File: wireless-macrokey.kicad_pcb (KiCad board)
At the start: 2 copper layers, 110.3 x 93.4 mm, 25 parts, among them J1 ENC0, J2 ENC1, J3 ENC2, J4 OLED, J5 POWER 5V, J6 SERIAL, J7 LED, SW1 SW_Push_45deg, SW10 SW_Push_45deg, SW11 SW_Push_45deg, SW12 SW_Push_45deg, SW13 SW_Push_45deg, SW14 SW_Push_45deg, SW2 SW_Push_45deg, SW3 SW_Push_45deg, SW4 SW_Push_45deg, SW5 SW_Push_45deg, SW6 SW_Push_45deg, SW7 SW_Push_45deg, SW8 SW_Push_45deg, SW9 SW_Push_45deg, U1 ESP32-WROOM-32E, U3 LM1117T-3.3

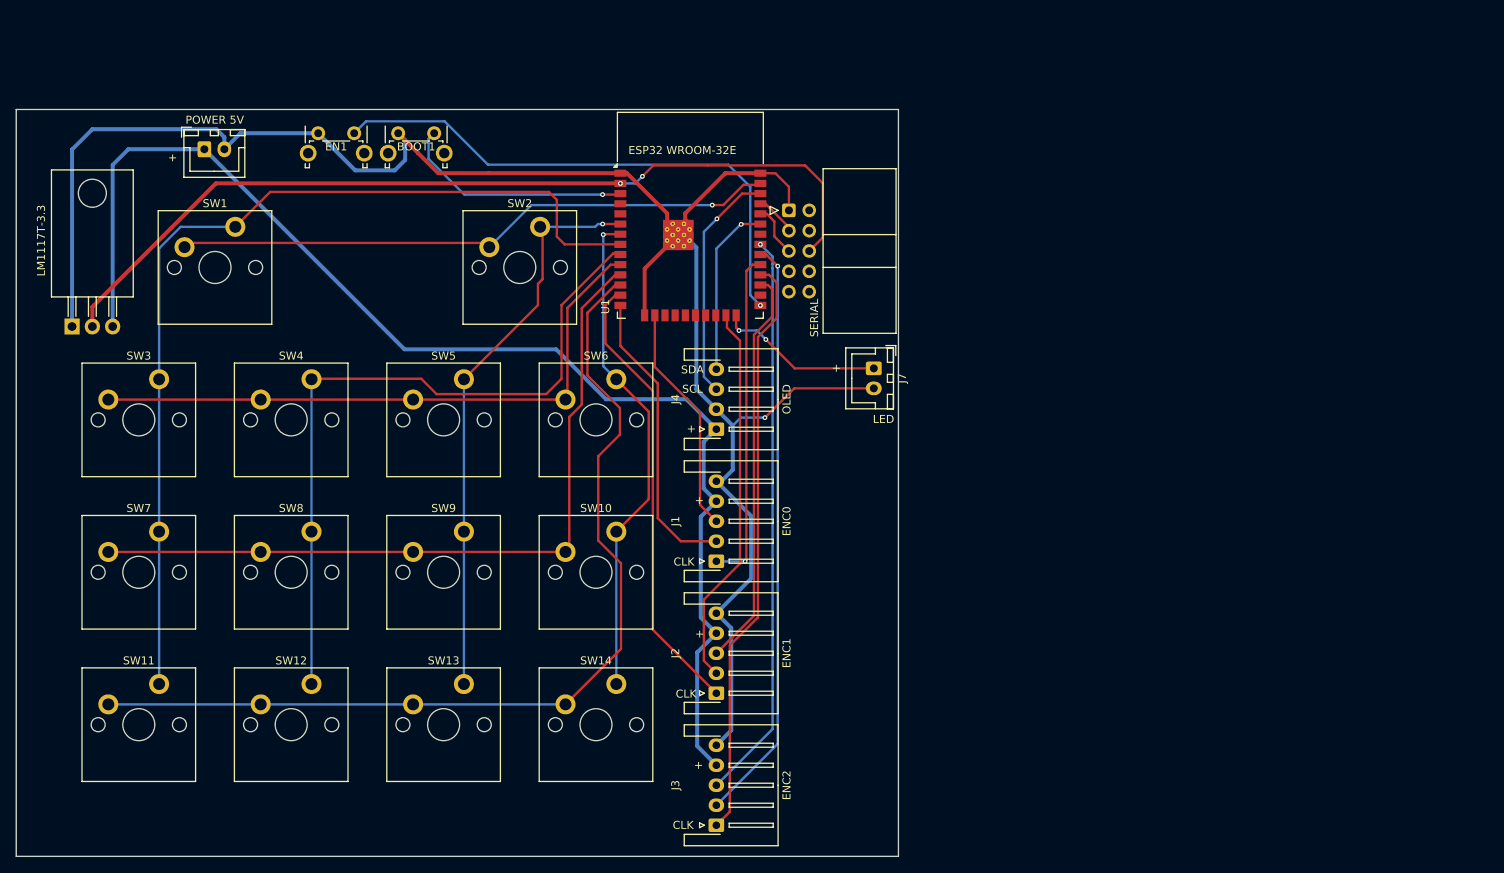
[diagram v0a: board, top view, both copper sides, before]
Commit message: x
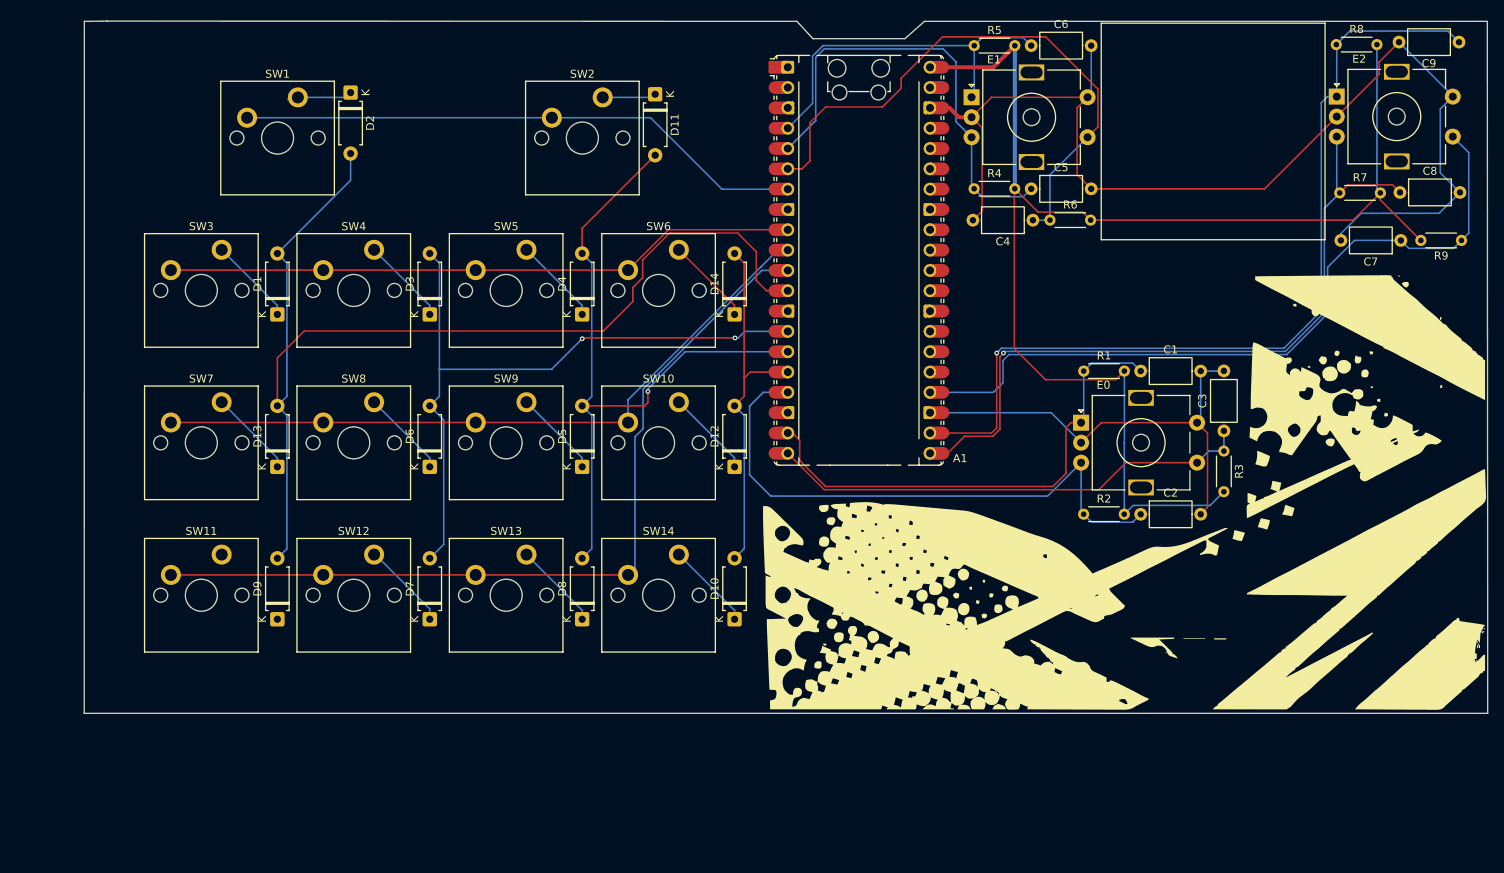
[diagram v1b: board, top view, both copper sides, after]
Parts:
- removed BOOT1, EN1: SW_Push, Button_Switch_THT:SW_Tactile_SPST_Angled_PTS645Vx39-2LFS
- removed J1: ENC0, Connector_JST:JST_XH_S5B-XH-A-1_1x05_P2.50mm_Horizontal
- removed J2: ENC1, Connector_JST:JST_XH_S5B-XH-A-1_1x05_P2.50mm_Horizontal
- removed J3: ENC2, Connector_JST:JST_XH_S5B-XH-A-1_1x05_P2.50mm_Horizontal
- removed J4: OLED, Connector_JST:JST_XH_S4B-XH-A-1_1x04_P2.50mm_Horizontal
- removed J5: POWER 5V, Connector_JST:JST_XH_B2B-XH-A_1x02_P2.50mm_Vertical
- removed J6: SERIAL, Connector_IDC:IDC-Header_2x05_P2.54mm_Horizontal
- removed J7: LED, Connector_JST:JST_XH_B2B-XH-A_1x02_P2.50mm_Vertical
- removed U1: ESP32-WROOM-32E, RF_Module:ESP32-WROOM-32D
- removed U3: LM1117T-3.3, Package_TO_SOT_THT:TO-220-3_Horizontal_TabDown
- added A1: RaspberryPi_Pico, Module:RaspberryPi_Pico_Common_Unspecified, F.Cu at (129.8, 53.4)
- added C1: 1uF, Capacitor_THT:C_Axial_L5.1mm_D3.1mm_P7.50mm_Horizontal, F.Cu at (165.0, 67.2)
- added C2: 1uF, Capacitor_THT:C_Axial_L5.1mm_D3.1mm_P7.50mm_Horizontal, F.Cu at (165.0, 85.1)
- added C3: 1uF, Capacitor_THT:C_Axial_L5.1mm_D3.1mm_P7.50mm_Horizontal, F.Cu at (175.4, 74.7)
- added C4: 1uF, Capacitor_THT:C_Axial_L5.1mm_D3.1mm_P7.50mm_Horizontal, F.Cu at (151.6, 48.4)
- added C5: 1uF, Capacitor_THT:C_Axial_L5.1mm_D3.1mm_P7.50mm_Horizontal, F.Cu at (151.3, 44.5)
- added C6: 1uF, Capacitor_THT:C_Axial_L5.1mm_D3.1mm_P7.50mm_Horizontal, F.Cu at (151.3, 26.6)
- added C7: 1uF, Capacitor_THT:C_Axial_L5.1mm_D3.1mm_P7.50mm_Horizontal, F.Cu at (197.6, 50.9)
- added C8: 1uF, Capacitor_THT:C_Axial_L5.1mm_D3.1mm_P7.50mm_Horizontal, F.Cu at (197.4, 44.9)
- added C9: 1uF, Capacitor_THT:C_Axial_L5.1mm_D3.1mm_P7.50mm_Horizontal, F.Cu at (204.8, 26.1)
- added D1: D_45deg, Diode_THT:D_A-405_P7.62mm_Horizontal, F.Cu at (57.1, 60.1)
- added D10: D_45deg, Diode_THT:D_A-405_P7.62mm_Horizontal, F.Cu at (114.3, 98.2)
- added D11: D_45deg, Diode_THT:D_A-405_P7.62mm_Horizontal, F.Cu at (104.3, 32.6)
- added D12: D_45deg, Diode_THT:D_A-405_P7.62mm_Horizontal, F.Cu at (114.3, 79.2)
- added D13: D_45deg, Diode_THT:D_A-405_P7.62mm_Horizontal, F.Cu at (57.1, 79.2)
- added D14: D_45deg, Diode_THT:D_A-405_P7.62mm_Horizontal, F.Cu at (114.3, 60.1)
- added D2: D_45deg, Diode_THT:D_A-405_P7.62mm_Horizontal, F.Cu at (66.3, 32.4)
- added D3: D_45deg, Diode_THT:D_A-405_P7.62mm_Horizontal, F.Cu at (76.2, 60.1)
- added D4: D_45deg, Diode_THT:D_A-405_P7.62mm_Horizontal, F.Cu at (95.2, 60.1)
- added D5: D_45deg, Diode_THT:D_A-405_P7.62mm_Horizontal, F.Cu at (95.2, 79.2)
- added D6: D_45deg, Diode_THT:D_A-405_P7.62mm_Horizontal, F.Cu at (76.2, 79.2)
- added D7: D_45deg, Diode_THT:D_A-405_P7.62mm_Horizontal, F.Cu at (76.2, 98.2)
- added D8: D_45deg, Diode_THT:D_A-405_P7.62mm_Horizontal, F.Cu at (95.2, 98.2)
- added D9: D_45deg, Diode_THT:D_A-405_P7.62mm_Horizontal, F.Cu at (57.1, 98.2)
- added E0: RotaryEncoder_Switch_MP, Rotary_Encoder:RotaryEncoder_Alps_EC11E-Switch_Vertical_H20mm_MountingHoles, F.Cu at (157.6, 73.7)
- added E1: RotaryEncoder_Switch_MP, Rotary_Encoder:RotaryEncoder_Alps_EC11E-Switch_Vertical_H20mm_MountingHoles, F.Cu at (143.9, 33.0)
- added E2: RotaryEncoder_Switch_MP, Rotary_Encoder:RotaryEncoder_Alps_EC11E-Switch_Vertical_H20mm_MountingHoles, F.Cu at (189.6, 32.9)
- added R1: 1k, Resistor_THT:R_Axial_DIN0204_L3.6mm_D1.6mm_P5.08mm_Horizontal, F.Cu at (157.9, 67.2)
- added R2: 1k, Resistor_THT:R_Axial_DIN0204_L3.6mm_D1.6mm_P5.08mm_Horizontal, F.Cu at (157.9, 85.1)
- added R3: 1k, Resistor_THT:R_Axial_DIN0204_L3.6mm_D1.6mm_P5.08mm_Horizontal, F.Cu at (175.4, 77.2)
- added R4: 1k, Resistor_THT:R_Axial_DIN0204_L3.6mm_D1.6mm_P5.08mm_Horizontal, F.Cu at (144.2, 44.4)
- added R5: 1k, Resistor_THT:R_Axial_DIN0204_L3.6mm_D1.6mm_P5.08mm_Horizontal, F.Cu at (144.2, 26.6)
- added R6: 1k, Resistor_THT:R_Axial_DIN0204_L3.6mm_D1.6mm_P5.08mm_Horizontal, F.Cu at (153.7, 48.4)
- added R7: 1k, Resistor_THT:R_Axial_DIN0204_L3.6mm_D1.6mm_P5.08mm_Horizontal, F.Cu at (189.9, 45.0)
- added R8: 1k, Resistor_THT:R_Axial_DIN0204_L3.6mm_D1.6mm_P5.08mm_Horizontal, F.Cu at (189.5, 26.4)
- added R9: 1k, Resistor_THT:R_Axial_DIN0204_L3.6mm_D1.6mm_P5.08mm_Horizontal, F.Cu at (205.1, 50.9)
- SW1, SW2: footprint PCM_Switch_Keyboard_Cherry_MX:SW_Cherry_MX_PCB_1.00u -> PCM_Switch_Keyboard_Cherry_MX:SW_Cherry_MX_PCB_2.00u
- moved SW14 18.0 mm to (104.8, 95.2)
- moved SW11 18.0 mm to (47.6, 95.2)
- moved SW12 18.0 mm to (66.7, 95.2)
- moved SW13 18.0 mm to (85.7, 95.2)
- moved SW6 18.0 mm to (104.8, 57.1)
- moved SW1 18.0 mm to (57.1, 38.1)
- moved SW3 18.0 mm to (47.6, 57.1)
- moved SW4 18.0 mm to (66.7, 57.1)
- moved SW10 18.0 mm to (104.8, 76.2)
- moved SW2 18.0 mm to (95.2, 38.1)
- moved SW5 18.0 mm to (85.7, 57.1)
- moved SW7 18.0 mm to (47.6, 76.2)
- moved SW8 18.0 mm to (66.7, 76.2)
- moved SW9 18.0 mm to (85.7, 76.2)
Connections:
- SW1 pad 2: Y1 -> Net-(D2-K)
- SW10 pad 2: Y4 -> Net-(D12-K)
- SW11 pad 2: Y1 -> Net-(D9-K)
- SW12 pad 2: Y2 -> Net-(D7-K)
- SW13 pad 2: Y3 -> Net-(D8-K)
- SW14 pad 2: Y4 -> Net-(D10-K)
- SW2 pad 2: Y3 -> Net-(D11-K)
- SW3 pad 2: Y1 -> Net-(D1-K)
- SW4 pad 2: Y2 -> Net-(D3-K)
- SW5 pad 2: Y3 -> Net-(D4-K)
- SW6 pad 2: Y4 -> Net-(D14-K)
- SW7 pad 2: Y1 -> Net-(D13-K)
- SW8 pad 2: Y2 -> Net-(D6-K)
- SW9 pad 2: Y3 -> Net-(D5-K)
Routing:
- net +3.3V: track 111.3 -> 0.00 mm, vias 2 -> 0
- net BOOT: track 68.9 -> 0.00 mm, vias 1 -> 0
- net DT2: track 73.3 -> 111.3 mm
- net GND: track 234.1 -> 200.5 mm, vias 1 -> 0
- net ESW0: track 29.8 -> 60.9 mm
- net CLK0: track 42.1 -> 72.9 mm, vias 1 -> 0
- net EN: track 29.4 -> 0.00 mm, vias 1 -> 0
- net SCL: track 29.4 -> 0.00 mm, vias 1 -> 0
- net DT0: track 37.1 -> 62.1 mm
- net ESW2: track 71.2 -> 94.3 mm, vias 1 -> 0
- net ESW1: track 50.1 -> 72.8 mm
- net SDA: track 21.8 -> 0.00 mm, vias 1 -> 0
- net LED: track 20.9 -> 0.00 mm, vias 2 -> 0
- net CLK2: track 73.4 -> 92.4 mm, vias 0 -> 1
- net Y1: track 120.4 -> 139.3 mm
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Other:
- board size 110.3 x 93.4 mm -> 175.4 x 86.5 mm
- board text removed: "+"
- board text removed: "CLK"
- board text removed: "ESP32 WROOM-32E"
- board text removed: "SCL"
- board text removed: "SDA"
